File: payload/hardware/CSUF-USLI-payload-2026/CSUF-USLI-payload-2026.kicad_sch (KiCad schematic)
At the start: 24 parts, among them U1 DEV-16771, U2 GPS6MV2, U3 MPU6050, U4 Adafruit BMP390, U5 RYLR896, U6 Generic RS485 to UART, U7 DF Robot EC and pH Placeholder

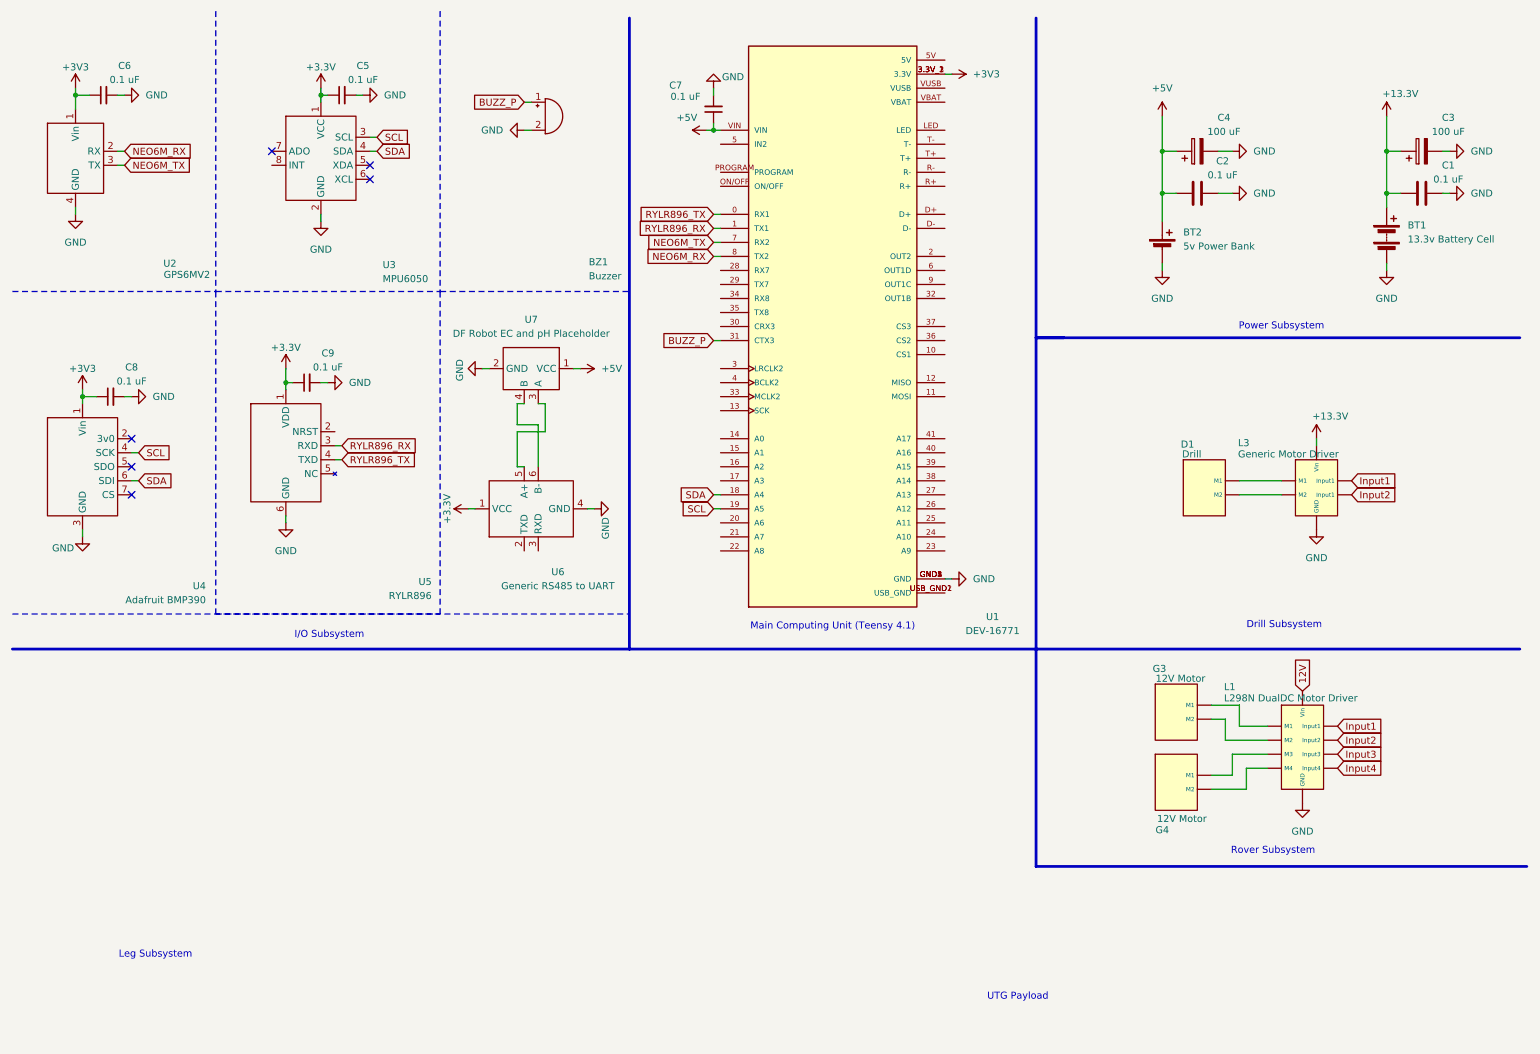
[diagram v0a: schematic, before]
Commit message: Update CSUF-USLI-payload-2026.kicad_sch
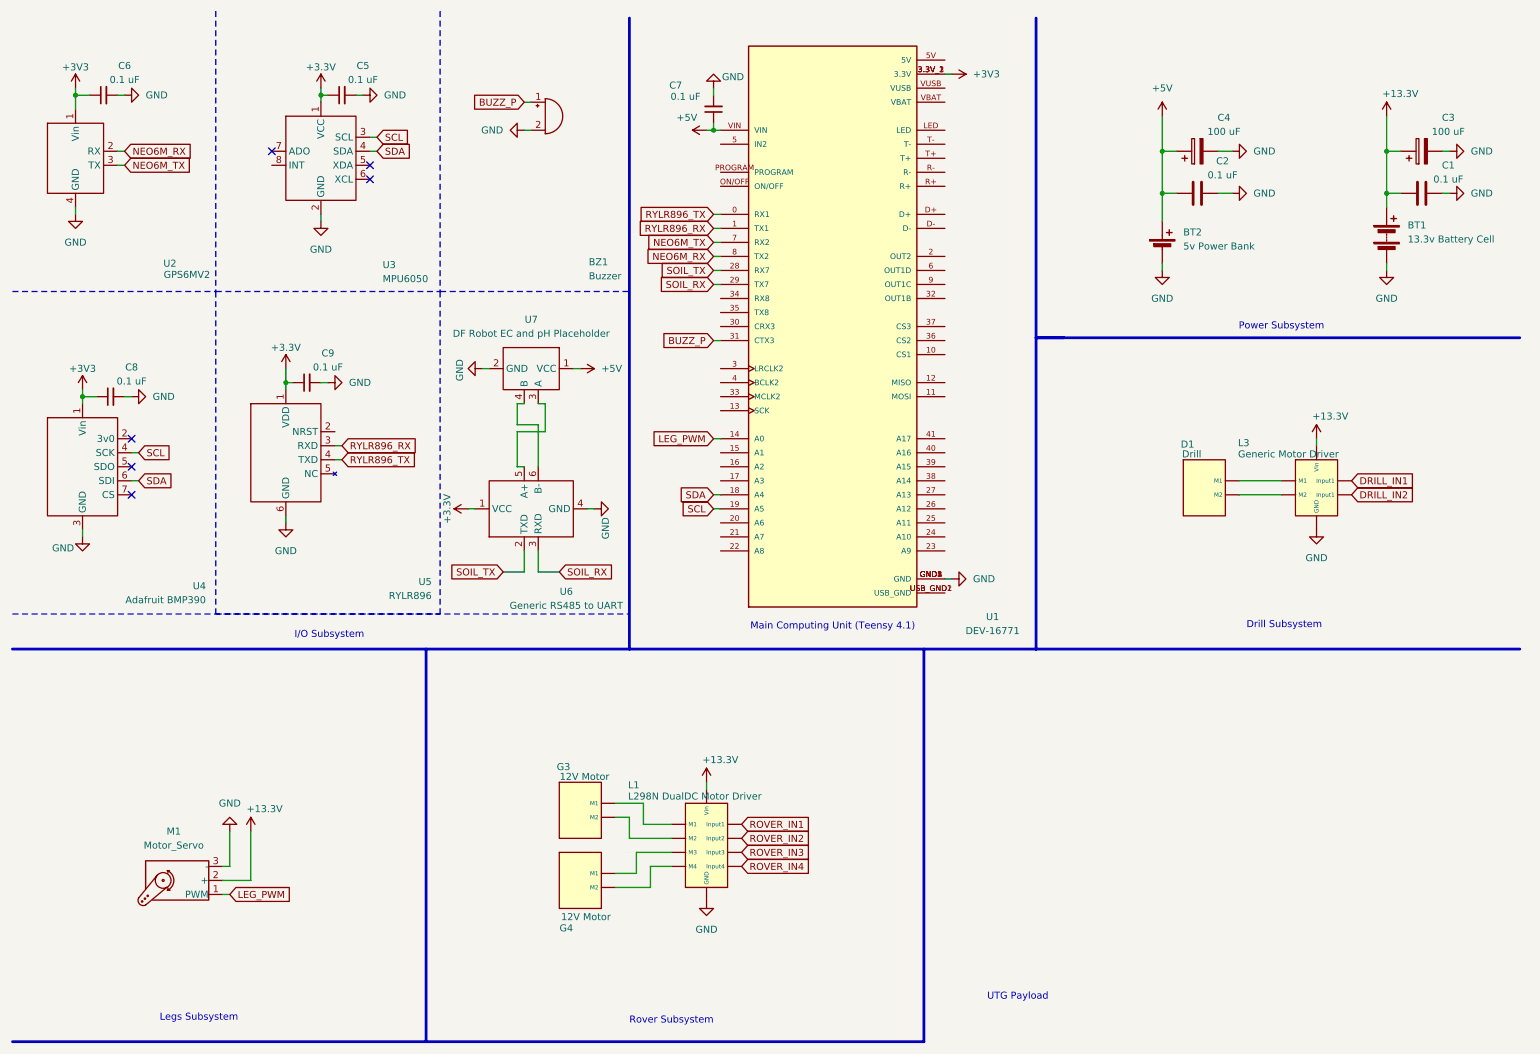
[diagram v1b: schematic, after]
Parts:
- added M1: Motor_Servo, symbol Motor:Motor_Servo
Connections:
- net 12V is gone; now on net ROVER_IN4: L1. (Input4)
- net Input3 is gone; now on net ROVER_IN4: L1. (Input4)
- net Input4 is gone; now on net ROVER_IN4: L1. (Input4)
- net +13.3V: now also L1. (Input4), M1.2 (+)
- net GND: now also M1.3 (-)
- net LEG_PWM: now reaches U1.14 (A0)
- net LEG_PWM: now also M1.1 (PWM)
- net SOIL_TX: now reaches U1.28 (RX7)
- net SOIL_TX: now also U6.2 (TXD)
- net SOIL_RX: now reaches U1.29 (TX7)
- net SOIL_RX: now also U6.3 (RXD)
- net ROVER_IN4: now reaches L1. (Input4)
- net ROVER_IN4: no longer G3. (M2)
- removed net Input1: L1. (Input4), L3. (Input1)
- removed net Input2: L1. (Input4), L3. (Input1)
- new net: D1. (M2), L3. (Input1)
- new net: G3. (M2), L1. (Input4)
- new net: G4. (M2), L1. (Input4)
- new net DRILL_IN1: L3. (Input1)
- new net DRILL_IN2: L3. (Input1)
- new net ROVER_IN1: L1. (Input4)
- new net ROVER_IN2: L1. (Input4)
- new net ROVER_IN3: L1. (Input4)
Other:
- note added: "Legs Subsystem"
- note removed: "Leg Subsystem"
- moved on the sheet: G3, G4, L1
